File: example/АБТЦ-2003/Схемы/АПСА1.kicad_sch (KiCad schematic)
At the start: 45 parts

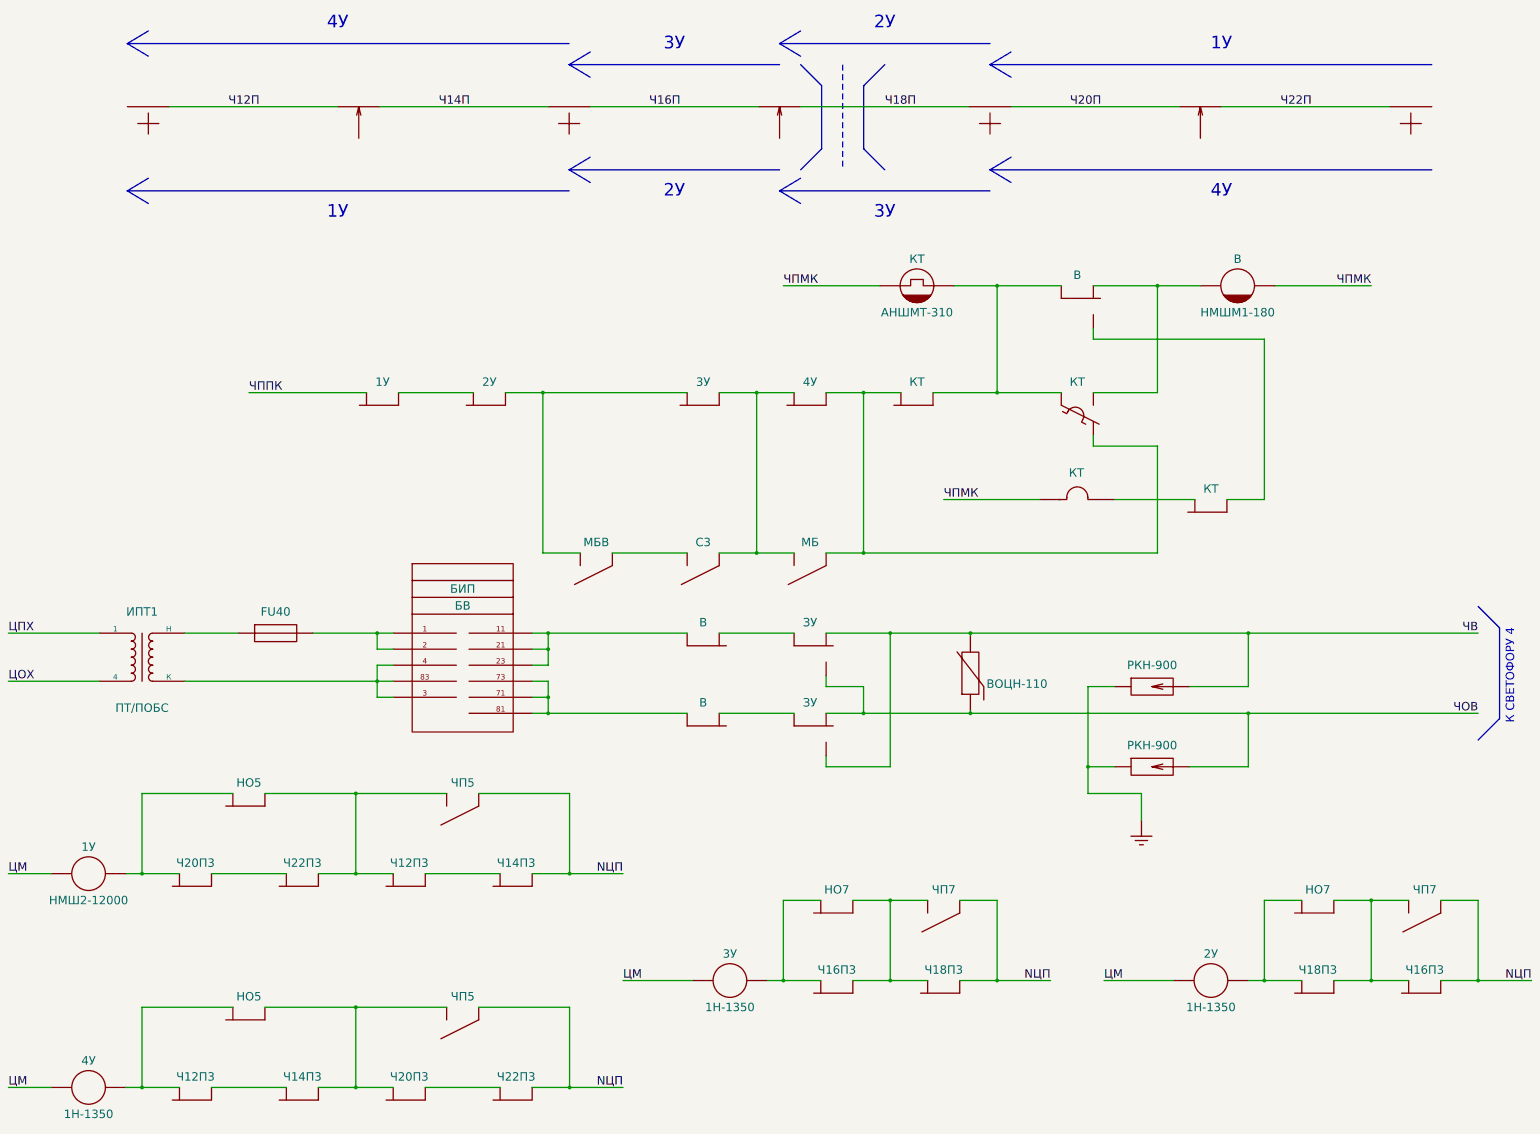
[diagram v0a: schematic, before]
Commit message: Шаблон АБТЦ обновлен
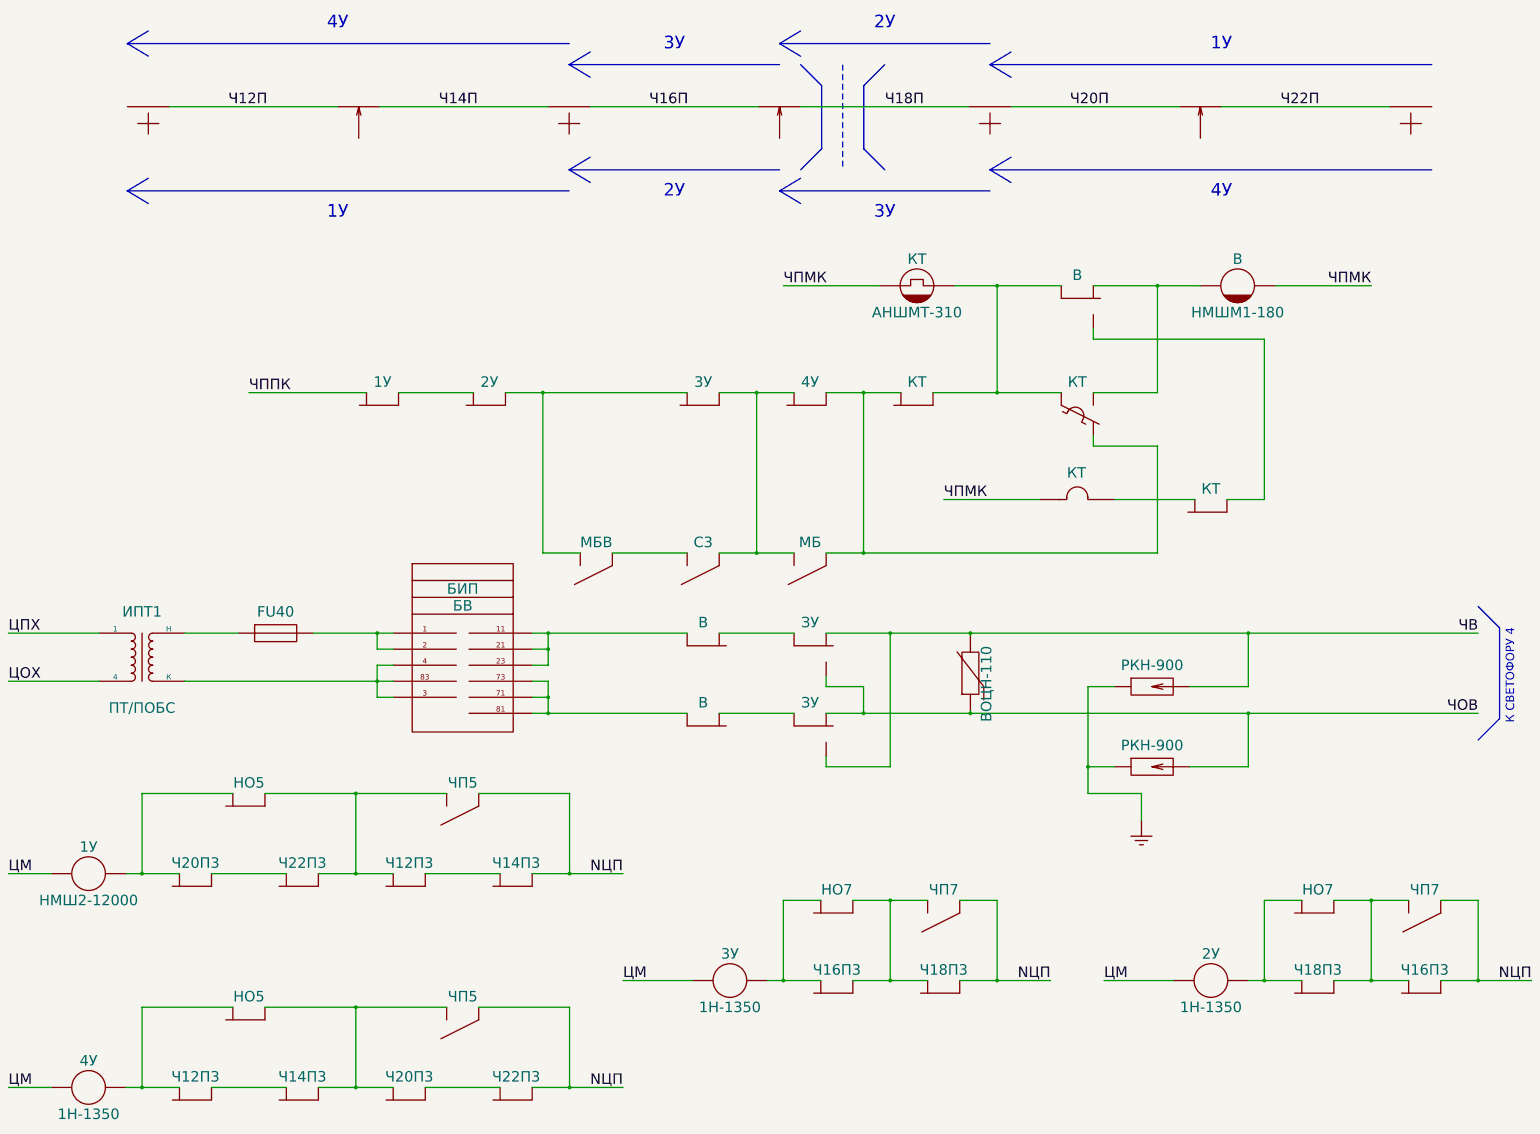
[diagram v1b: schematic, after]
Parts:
- Генератор1, Генератор11, Генератор111: symbol SCB:Генератор_Нитки -> SCB_АБТЦ:Генератор_Нитки
- Приемник1, Приемник11, Приемник111: symbol SCB:Приемник_Нитки -> SCB_АБТЦ:Приемник_Нитки

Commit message: Обновление примера
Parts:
- Н11, Н111, Н1111, Н11111, Н111111, Н1111111, Н11112, Н111121, Н14: symbol SCB_Relay:Контакт_нейтрального_якоря_НЗ -> SCB_Legacy:Контакт_нейтрального_якоря_НЗ_бн
- Н11, Н11112, Н111121, Н1111211, Н12: symbol SCB_Relay:Контакт_нейтрального_якоря -> SCB_Legacy:Контакт_нейтрального_якоря_бн
